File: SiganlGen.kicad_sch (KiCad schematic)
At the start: 79 parts, among them J1 Barrel_Jack_MountingPin, J2 Conn_Coaxial, J3 Conn_01x08_Socket, Q1 BC557, Q2 BC547, SW1 RotaryEncoder_Switch, SW10 SW_Push_45deg, SW11 SW_Push_45deg, SW12 SW_Push_45deg, SW13 SW_Push_45deg, SW14 SW_Push_45deg, SW15 SW_Push_45deg, SW16 SW_Push_45deg, SW17 SW_Push_45deg, SW18 SW_Push, SW19 SW_Push, SW2 SW_Push_45deg, SW20 SW_Push, SW21 SW_Push, SW3 SW_Push_45deg, SW4 SW_Push_45deg, SW5 SW_Push_45deg, SW6 SW_Push_45deg, SW7 SW_Push_45deg, SW8 SW_Push_45deg, SW9 SW_Push_45deg, U1 RaspberryPi_Pico, U2 L7805, U3 NE5532, U4 MC34063AP, U5 NE5532, U6 LM7910_TO220, U7 LM7810_TO220

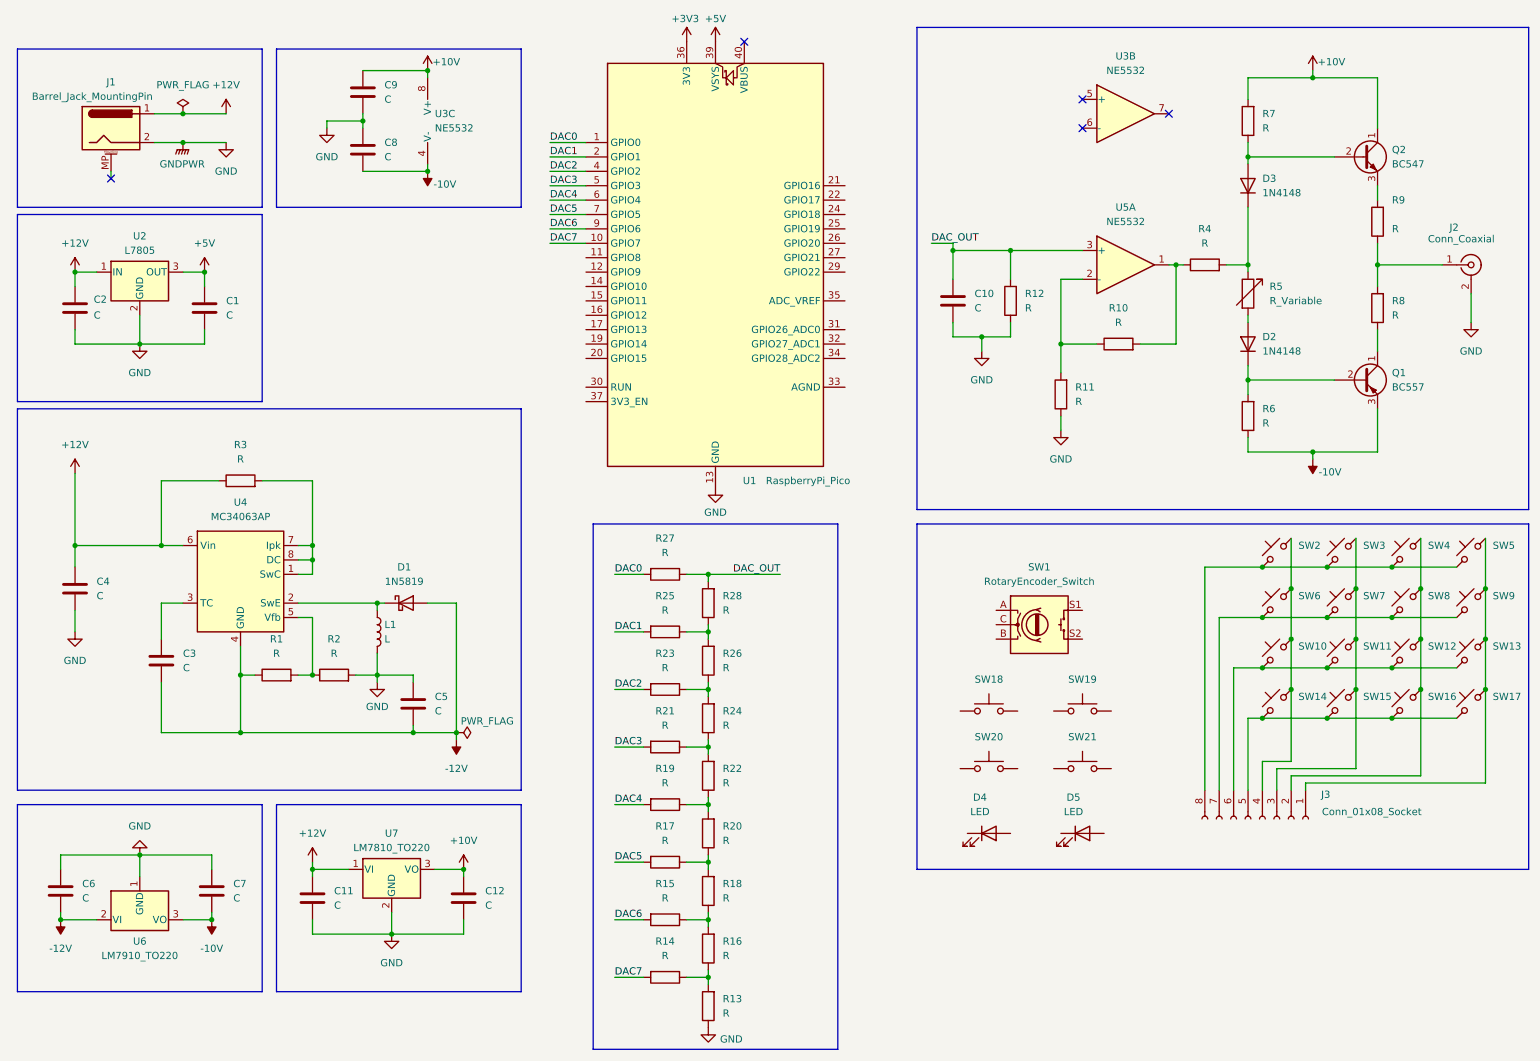
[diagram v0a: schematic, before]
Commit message: footprints
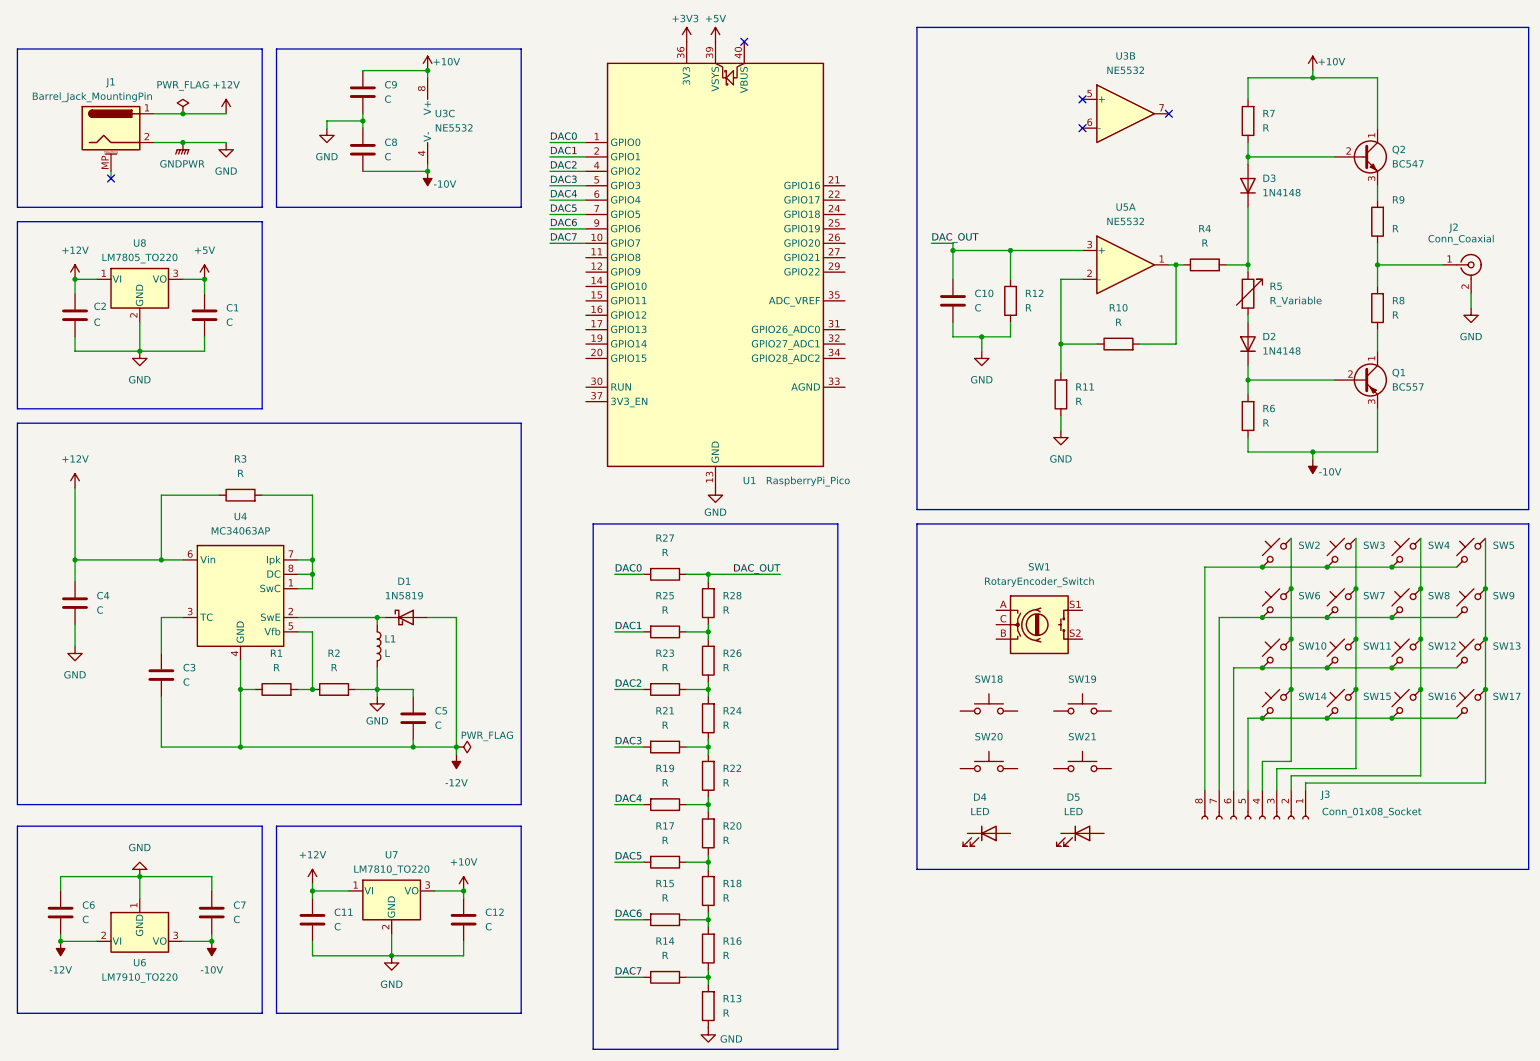
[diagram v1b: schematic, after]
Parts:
- removed U2: L7805, Package_TO_SOT_SMD:TO-252-3_TabPin2, symbol Regulator_Linear:L7805
- added U8: LM7805_TO220, Package_TO_SOT_THT:TO-220-3_Vertical, symbol Regulator_Linear:LM7805_TO220
- Q1: footprint Package_TO_SOT_THT:TO-92_Inline -> Package_TO_SOT_THT:TO-92_HandSolder
- U3, U5: footprint (none) -> Package_DIP:DIP-8_W7.62mm_Socket_LongPads
- U4: footprint Package_SO:SOIC-8_3.9x4.9mm_P1.27mm -> Package_DIP:DIP-8_W7.62mm_Socket_LongPads
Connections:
- net +12V: now also U8.1 (VI)
- net +5V: now also U8.3 (VO)
- net GND: now also U8.2 (GND)
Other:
- moved on the sheet: C1, C11, C12, C2, C3, C4, C5, C6, C7, D1, L1, R1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
